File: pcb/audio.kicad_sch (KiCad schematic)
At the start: 15 parts, among them J3 AudioJack4, U3 ES7210, U5 ES8311

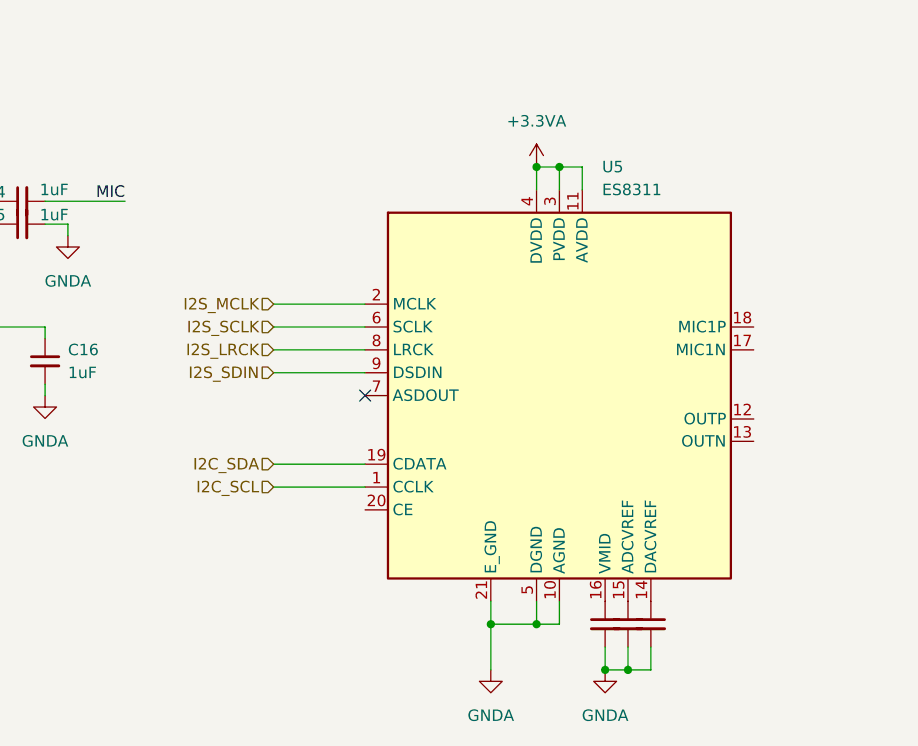
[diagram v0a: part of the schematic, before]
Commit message: caps
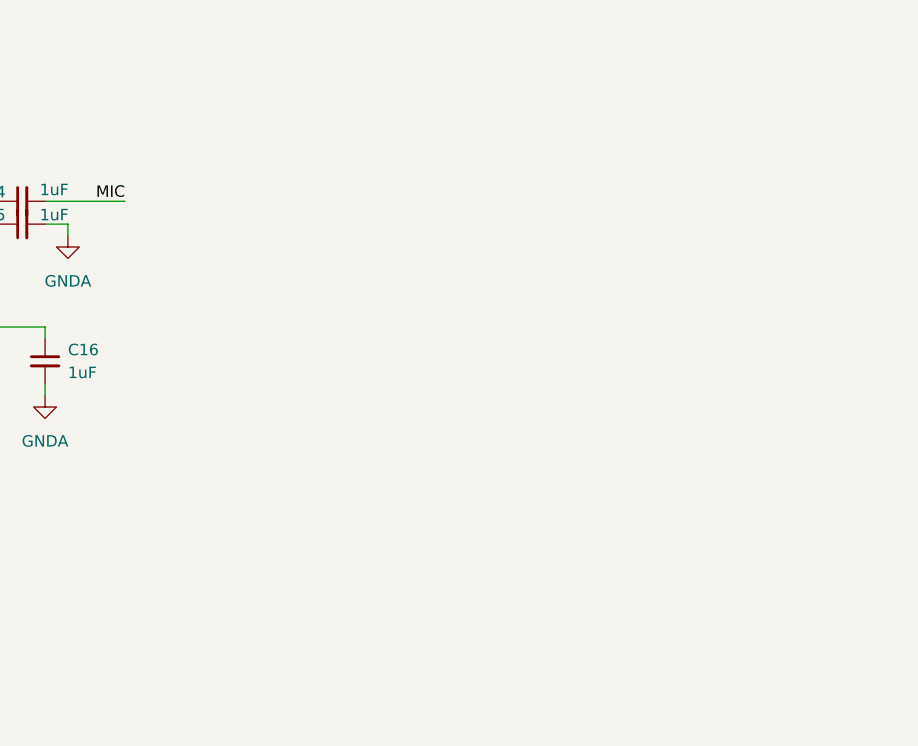
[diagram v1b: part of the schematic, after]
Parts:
- removed C19, C20, C21: 1uF, symbol Device:C_Small
- removed U5: ES8311, symbol live-caption-badge:ES8311
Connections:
- no-connect marks 10 -> 9
